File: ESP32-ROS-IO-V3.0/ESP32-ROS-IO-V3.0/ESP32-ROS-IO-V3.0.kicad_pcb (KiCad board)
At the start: 2 copper layers, 54 parts, among them J1 Conn_01x19_Socket, J10 XT30UPB-F, J11 XT30UPB-F, J12 XT30UPB-F, J13 XT30UPB-F, J14 XT30UPB-F, J15 XT30UPB-F, J16 XT60-M, J17 XT60-M, J2 Conn_01x19_Socket, J3 Conn_01x19_Socket, J4 Conn_01x19_Socket, J5 Conn_01x02_Pin, J6 Conn_01x02_Pin, J7 Conn_01x04_Socket, J8 XT30UPB-F, J9 XT30UPB-F, SW1 SW1, SW2 SW2, SW3 SW3, SW4 SW4, SW5 SW5, SW6 SW6, SW7 SW7, SW8 SW7

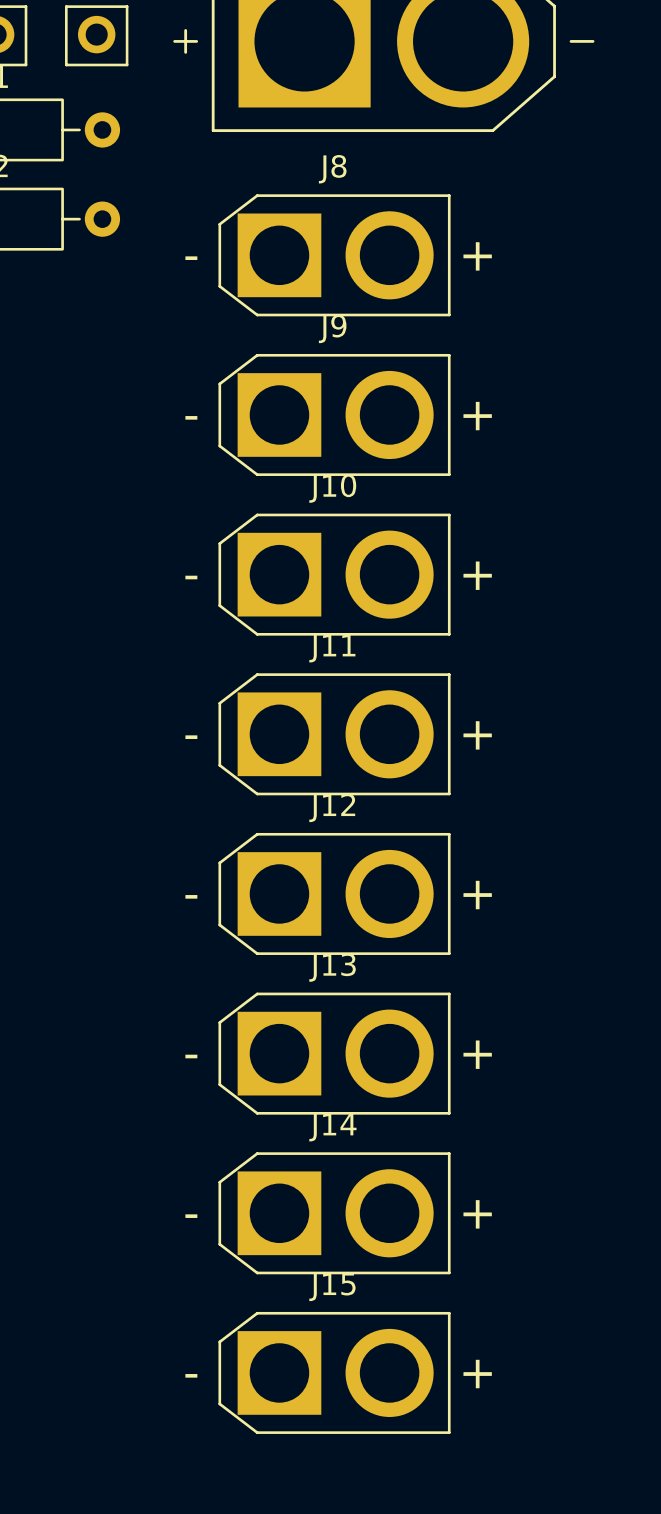
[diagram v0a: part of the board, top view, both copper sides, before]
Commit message: (T_T)
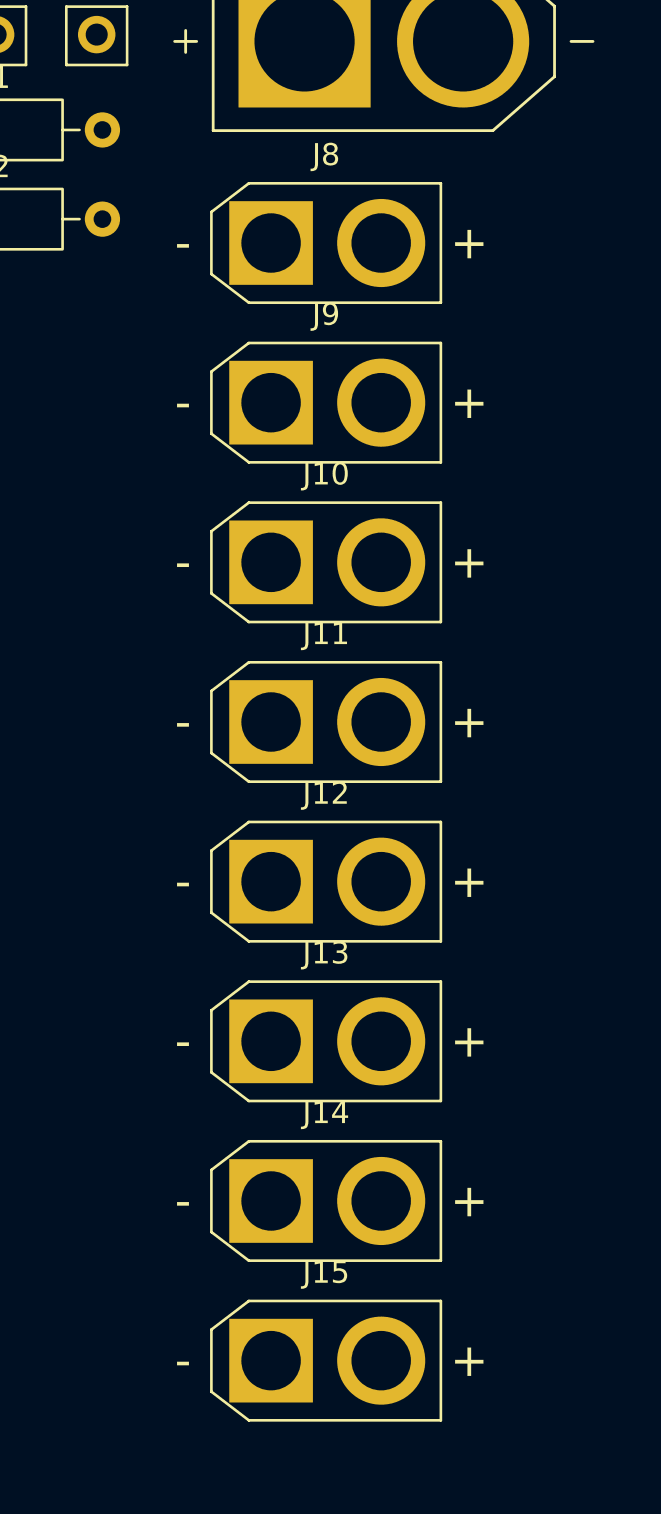
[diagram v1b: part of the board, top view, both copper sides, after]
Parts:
- moved J10 0.68 mm to (85.7, 111.6)
- moved J11 0.68 mm to (85.7, 118.8)
- moved J12 0.68 mm to (85.7, 126.1)
- moved J13 0.68 mm to (85.7, 133.3)
- moved J14 0.68 mm to (85.7, 140.6)
- moved J15 0.68 mm to (85.7, 147.8)
- moved J8 0.68 mm to (85.7, 97.1)
- moved J9 0.68 mm to (85.7, 104.3)
